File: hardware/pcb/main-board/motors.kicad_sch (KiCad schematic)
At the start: 31 parts, among them J12 Stepper JST, J13 Stepper JST, J14 CAN-FD Port, U6 DRV8436PWPR, U7 DRV8436PWPR, U9 ATA6563-GAQW1

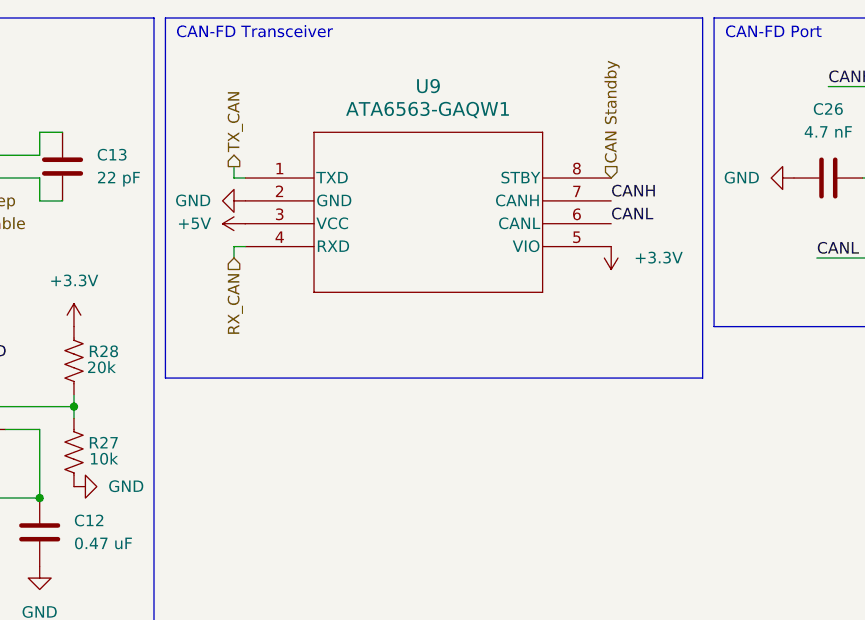
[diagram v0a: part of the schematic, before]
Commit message: RS485 Comms
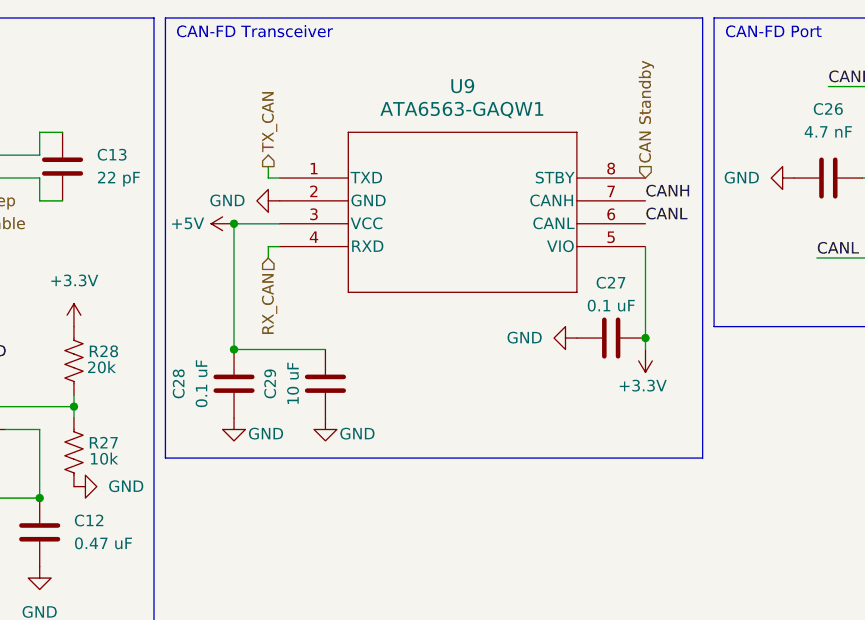
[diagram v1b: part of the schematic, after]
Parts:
- added C27, C28: 0.1 uF, symbol Device:C
- added C29: 10 uF, symbol Device:C
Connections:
- net +3.3V: now also C27.2
- net +5V: now also C28.2, C29.2
- net GND: now also C27.1, C28.1, C29.1
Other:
- moved on the sheet: U9
